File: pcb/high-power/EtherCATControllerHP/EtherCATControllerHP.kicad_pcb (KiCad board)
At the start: 6 copper layers, 77 x 77 mm, 181 parts, among them J1 DNP, J2 Right Angle 1x4, J3 Conn_01x04_Socket, J4 TYPE-C-31-M-12, J5 XT60PW-M, J6 2 pin Molex Picoblade, J7 DEBUG POWER, SW1 EVP-AA202K, U1 STM32F405RGT6, U2 TPS54360DDAR, U3 LDL1117S33R, U4 LAN9252I/ML, U5 AS5047P-ATSM, U6 MCF8329A1IREER, U7 24FC512-I/SN, U8 SN65HVD231, Y1 ABM3B-8.000MHZ-10-1-U-T, Y2 ABM8-25.000MHZ-D2Y-T

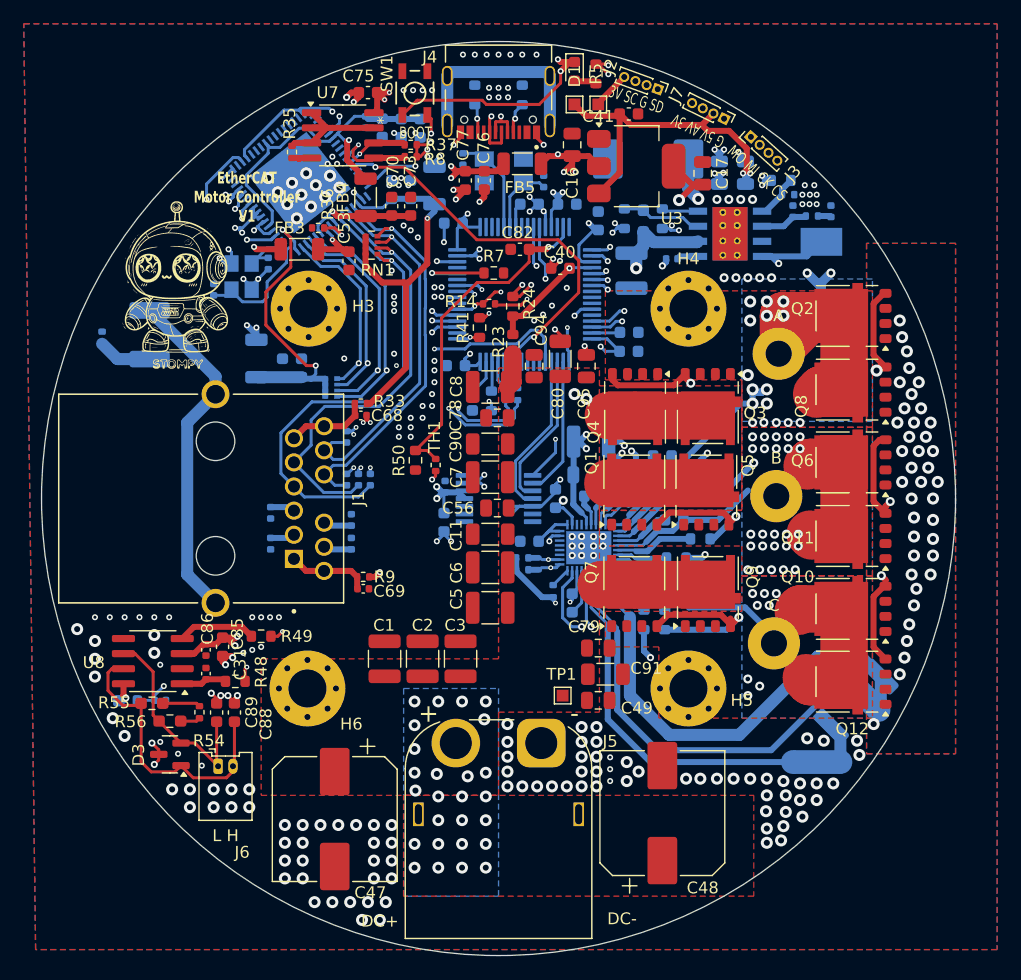
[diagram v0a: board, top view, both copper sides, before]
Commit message: production files
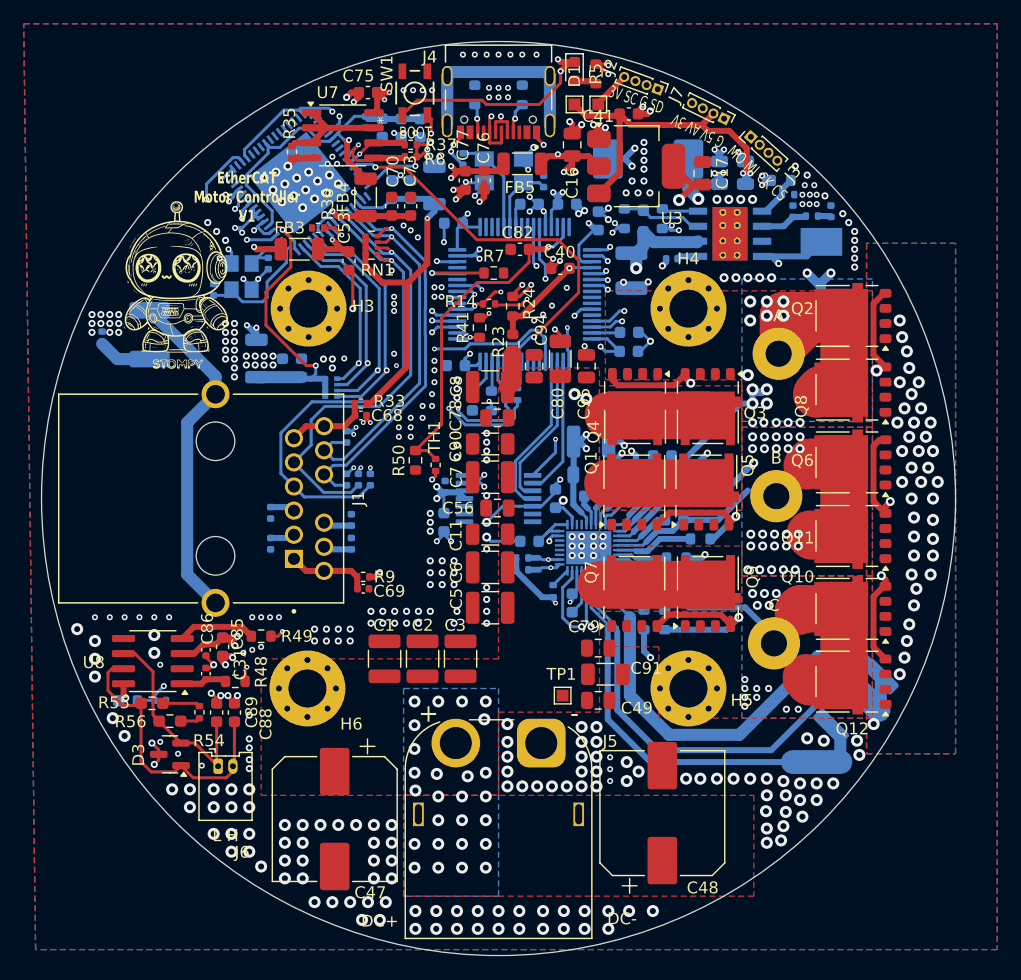
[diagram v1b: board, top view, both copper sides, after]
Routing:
- net GND: track 88.0 -> 129.5 mm, vias 277 -> 438
- net /SH_C: vias 8 -> 14
